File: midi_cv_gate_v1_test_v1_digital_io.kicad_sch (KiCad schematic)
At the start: 46 parts, among them U104 MCP23018_SP

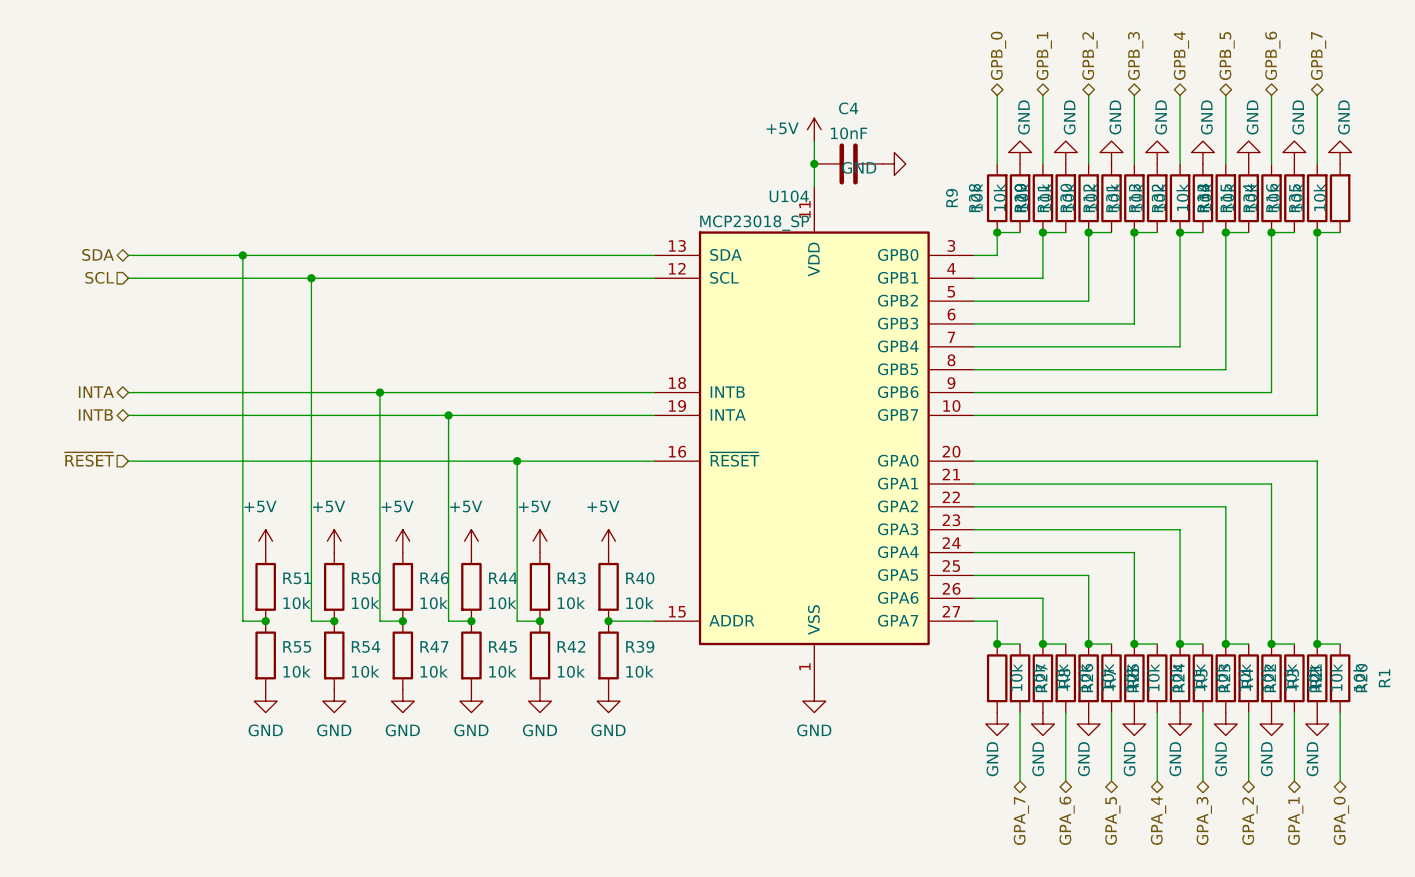
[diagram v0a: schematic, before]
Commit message: A little cleanup
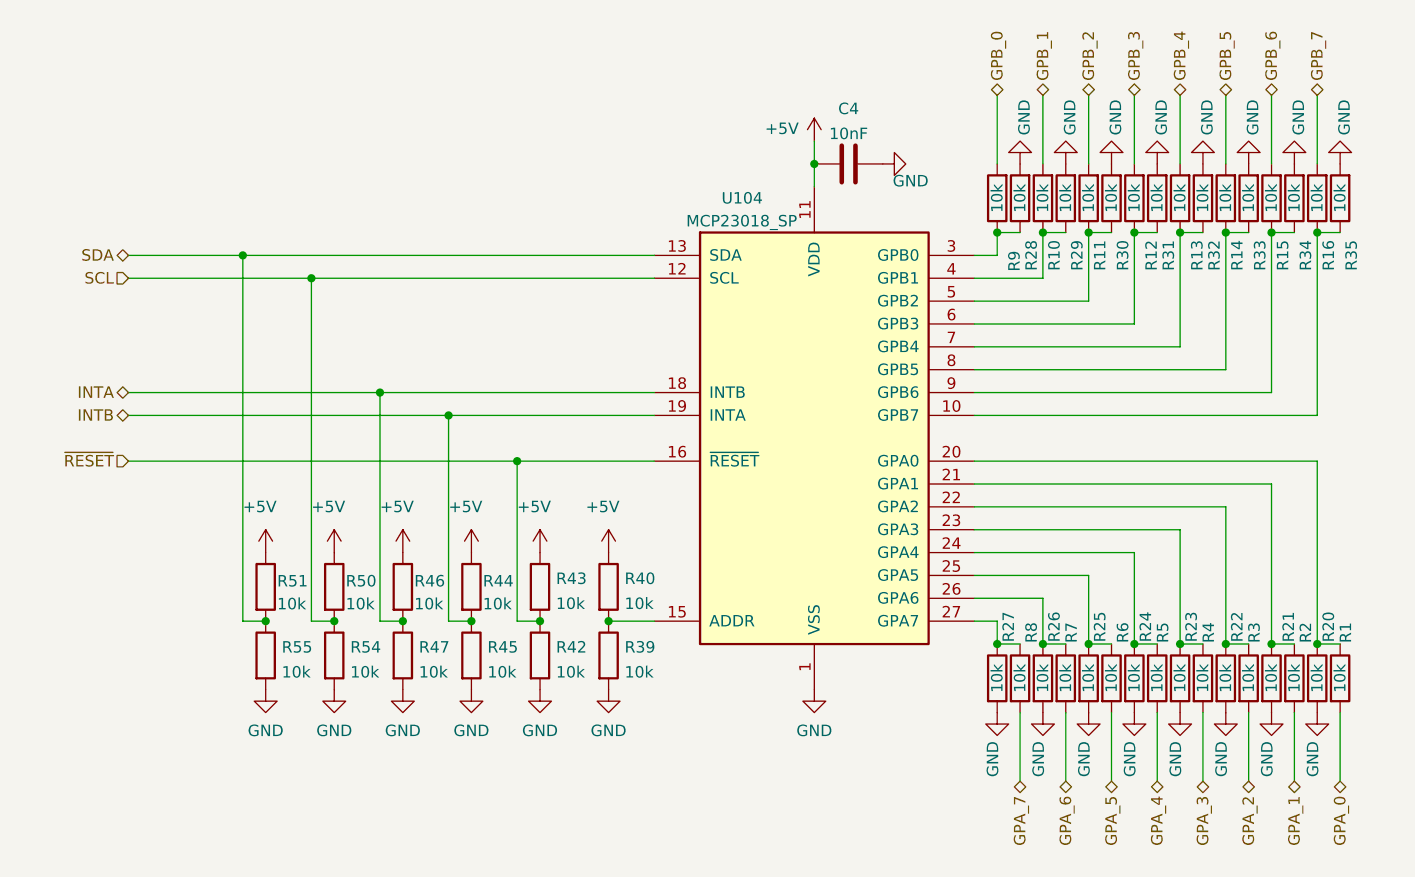
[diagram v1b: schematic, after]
